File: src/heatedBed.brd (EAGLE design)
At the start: 100 x 100 mm, 21 parts, among them P2 LONG_PAD

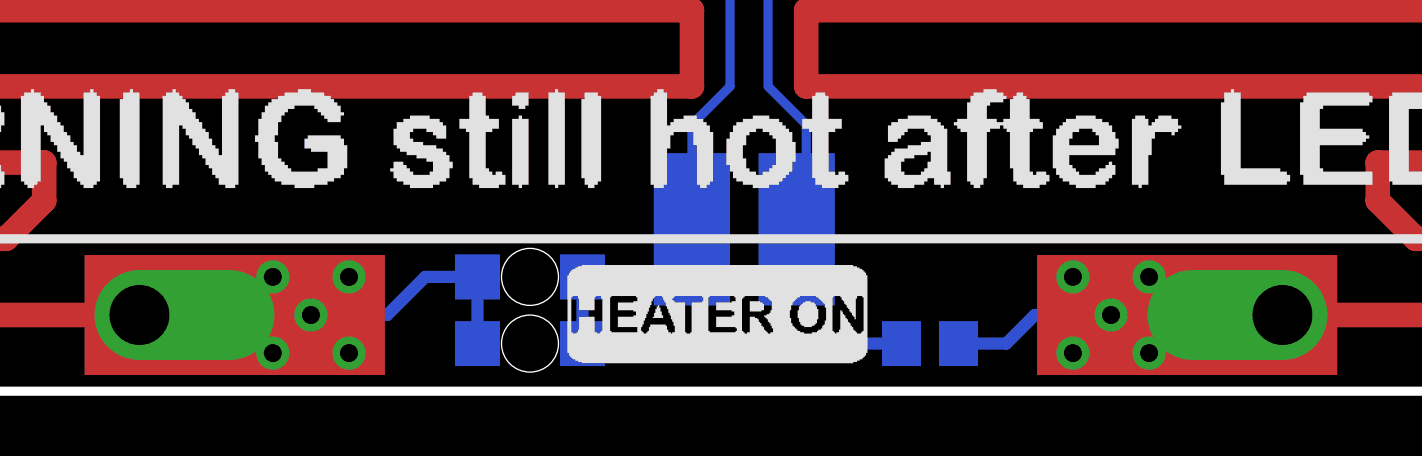
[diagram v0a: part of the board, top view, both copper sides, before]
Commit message: Updated revision B files.
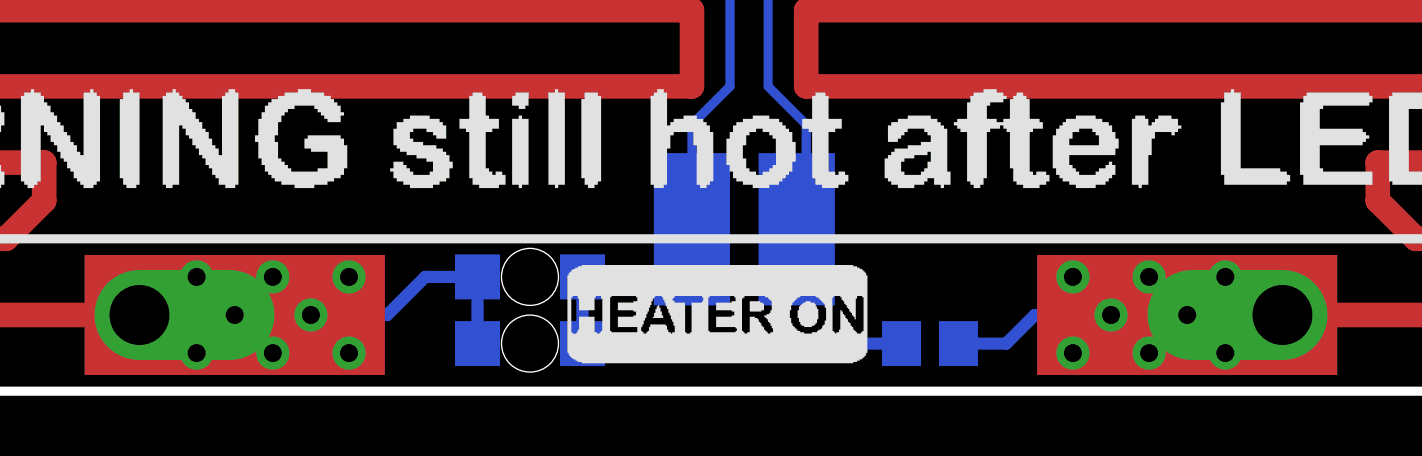
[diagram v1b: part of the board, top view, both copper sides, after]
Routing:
- net P1: vias 10 -> 16
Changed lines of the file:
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@@
 <?xml version="1.0" encoding="utf-8"?>
 <!DOCTYPE eagle SYSTEM "eagle.dtd">
-<eagle version="7.4.0">
+<eagle version="7.0.0">
 <drawing>
 <settings>
@@
 <layers>
 <layer number="1" name="Top" color="4" fill="1" visible="yes" active="yes"/>
-<layer number="16" name="Bottom" color="1" fill="1" visible="yes" active="yes"/>
+<layer number="16" name="Bottom" color="1" fill="1" visible="no" active="yes"/>
 <layer number="17" name="Pads" color="2" fill="1" visible="yes" active="yes"/>
 <layer number="18" name="Vias" color="2" fill="1" visible="yes" active="yes"/>
@@
 <via x="60.96" y="1.27" extent="1-16" drill="0.6"/>
 <via x="63.5" y="1.27" extent="1-16" drill="0.6"/>
+<via x="33.02" y="2.54" extent="1-16" drill="0.6"/>
+<via x="31.75" y="3.81" extent="1-16" drill="0.6"/>
+<via x="31.75" y="1.27" extent="1-16" drill="0.6"/>
+<via x="64.77" y="2.54" extent="1-16" drill="0.6"/>
+<via x="66.04" y="3.81" extent="1-16" drill="0.6"/>
+<via x="66.04" y="1.27" extent="1-16" drill="0.6"/>
+<wire x1="64.77" y1="2.54" x2="66.04" y2="3.81" width="0" layer="19" extent="16-16"/>
+<wire x1="63.5" y1="3.81" x2="64.77" y2="2.54" width="0" layer="19" extent="16-16"/>
+<wire x1="66.04" y1="1.27" x2="64.77" y2="2.54" width="0" layer="19" extent="16-16"/>
+<wire x1="60.96" y1="3.81" x2="59.69" y2="2.54" width="0" layer="19" extent="16-16"/>
 <wire x1="62.23" y1="2.54" x2="63.5" y2="3.81" width="0" layer="19" extent="1-1"/>
-<wire x1="60.96" y1="3.81" x2="62.23" y2="2.54" width="0" layer="19" extent="1-1"/>
-<wire x1="63.5" y1="1.27" x2="62.23" y2="2.54" width="0" layer="19" extent="1-1"/>
-<wire x1="60.96" y1="1.27" x2="62.23" y2="2.54" width="0" layer="19" extent="1-1"/>
-<wire x1="64.77" y1="2.54" x2="63.5" y2="3.81" width="0" layer="19" extent="16-16"/>
-<wire x1="64.77" y1="2.54" x2="64.77" y2="2.54" width="0" layer="19" extent="1-16"/>
-<wire x1="33.02" y1="2.54" x2="33.02" y2="2.54" width="0" layer="19" extent="1-16"/>
+<wire x1="63.5" y1="1.27" x2="64.77" y2="2.54" width="0" layer="19" extent="16-16"/>
+<wire x1="60.96" y1="1.27" x2="59.69" y2="2.54" width="0" layer="19" extent="16-16"/>
 <wire x1="36.83" y1="3.81" x2="38.1" y2="2.54" width="0" layer="19" extent="16-16"/>
 <wire x1="35.56" y1="2.54" x2="36.83" y2="3.81" width="0" layer="19" extent="1-1"/>
-<wire x1="34.29" y1="3.81" x2="33.02" y2="2.54" width="0" layer="19" extent="1-1"/>
+<wire x1="34.29" y1="3.81" x2="33.02" y2="2.54" width="0" layer="19" extent="16-16"/>
 <wire x1="36.83" y1="1.27" x2="38.1" y2="2.54" width="0" layer="19" extent="16-16"/>
-<wire x1="34.29" y1="1.27" x2="33.02" y2="2.54" width="0" layer="19" extent="1-1"/>
+<wire x1="34.29" y1="1.27" x2="33.02" y2="2.54" width="0" layer="19" extent="16-16"/>
+<wire x1="31.75" y1="3.81" x2="33.02" y2="2.54" width="0" layer="19" extent="16-16"/>
+<wire x1="31.75" y1="1.27" x2="33.02" y2="2.54" width="0" layer="19" extent="16-16"/>
 </signal>
 <signal name="N$4">
